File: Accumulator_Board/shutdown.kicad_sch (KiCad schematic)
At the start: 20 parts, among them J6 Shutdown IL, K1 DK1A1B-12V, K3 DK1A1B-12V, K4 G6BK-1114P-US, U11 SN74HCS08DR, U7 HEF4093B

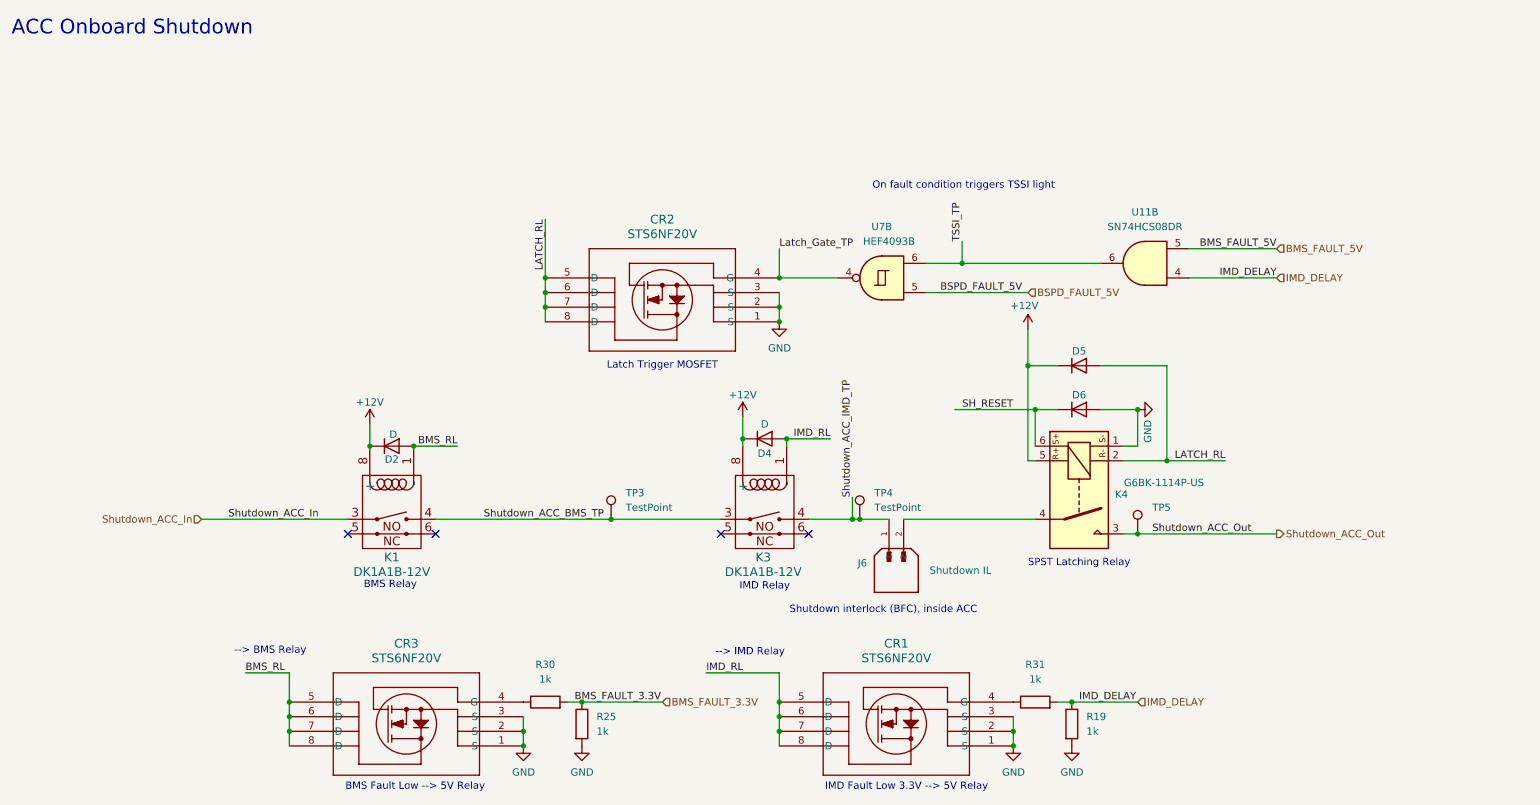
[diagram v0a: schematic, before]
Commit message: Acc Onboard Shutdown cleanup
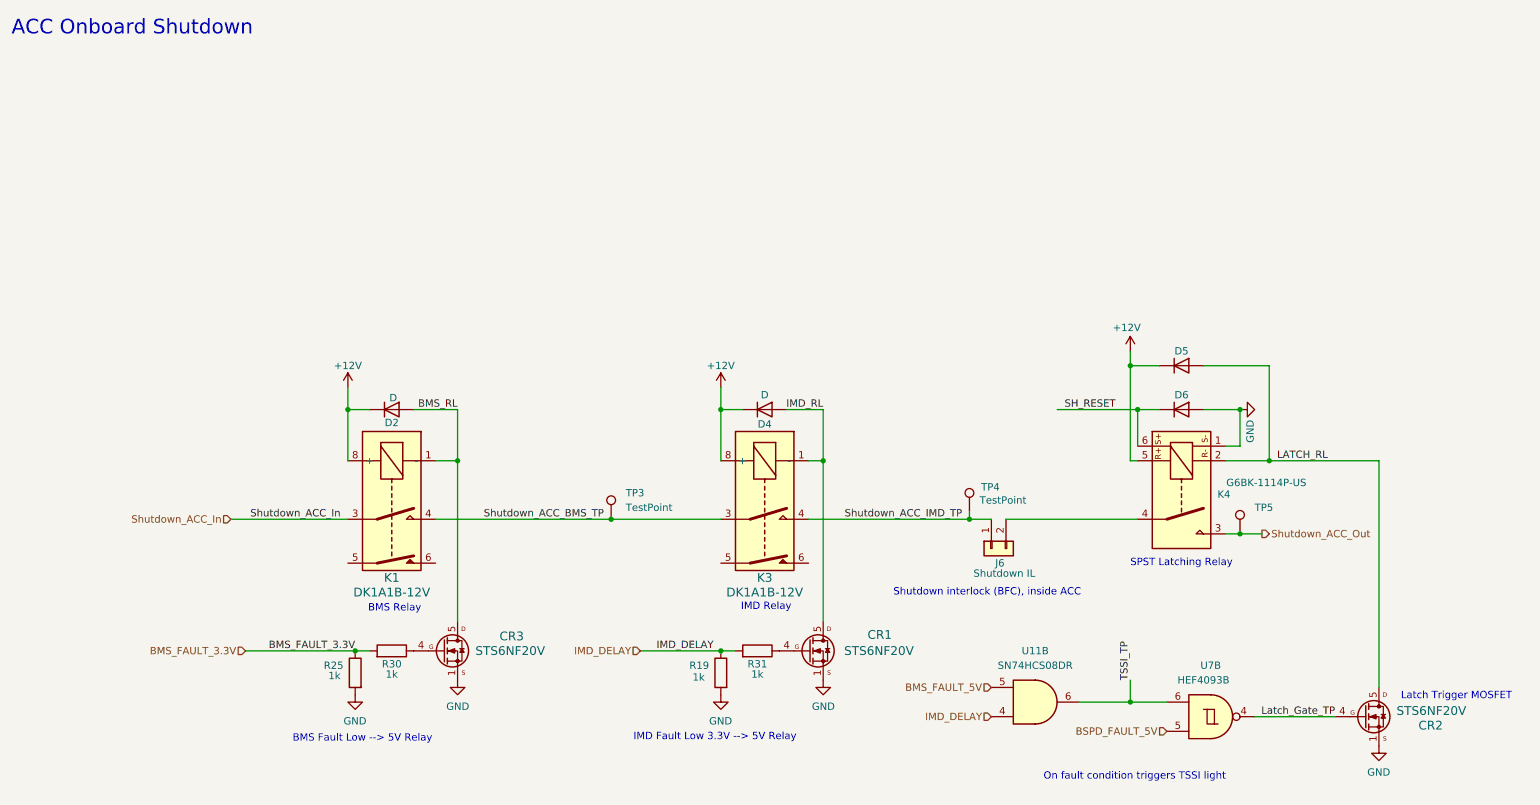
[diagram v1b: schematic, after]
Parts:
- CR1, CR2, CR3: symbol FS_2_Global_Symbol_Library:STS6NF20V -> FS_3_Global_Symbol_Library:STS6NF20V
- J6: symbol molex_1053091202:1053091202 -> Connector_Generic:Conn_01x02
- K1, K3: symbol 2FS-1_Symbol Library:DK1A1B-12V -> FS_3_Global_Symbol_Library:DK1A1B-12V
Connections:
- no-connect marks 4 -> 0
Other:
- note removed: "--> BMS Relay"
- note removed: "--> IMD Relay"
- moved on the sheet: D2, D4, D5, D6, K4, R19, R25, R30, R31, TP4, TP5, U11B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
